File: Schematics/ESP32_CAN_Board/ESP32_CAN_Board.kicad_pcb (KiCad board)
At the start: 4 copper layers, 56 x 50 mm, 36 parts, among them J1 Screw_Terminal_01x04, J2 Screw_Terminal_01x04, J3 Screw_Terminal_01x02, J8 USB_C_Receptacle, U1 SN65HVD230, U4 ESP32-C3-MINI-1-N4, U7 LDL1117-3.3

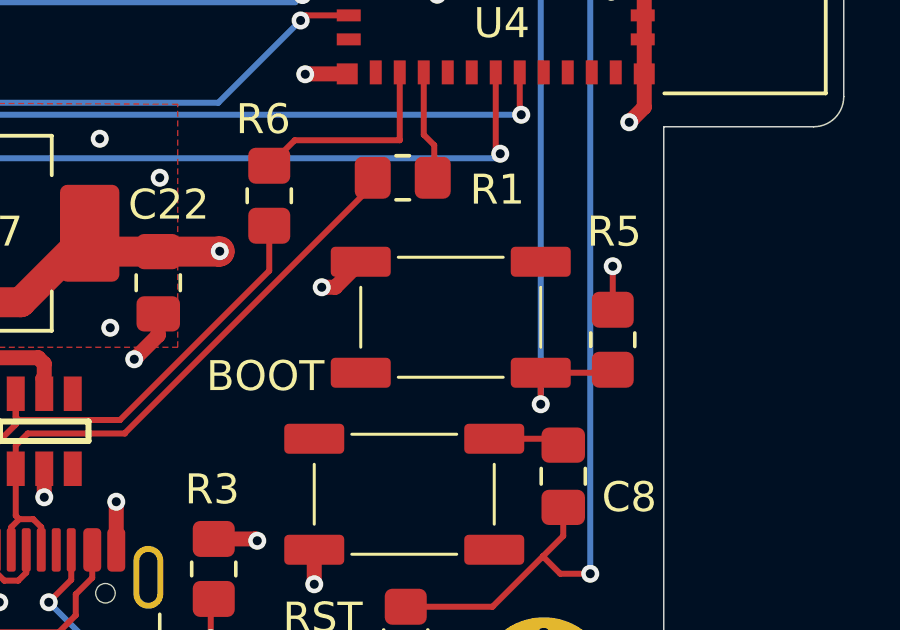
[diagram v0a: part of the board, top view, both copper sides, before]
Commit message: updated ESPBoard
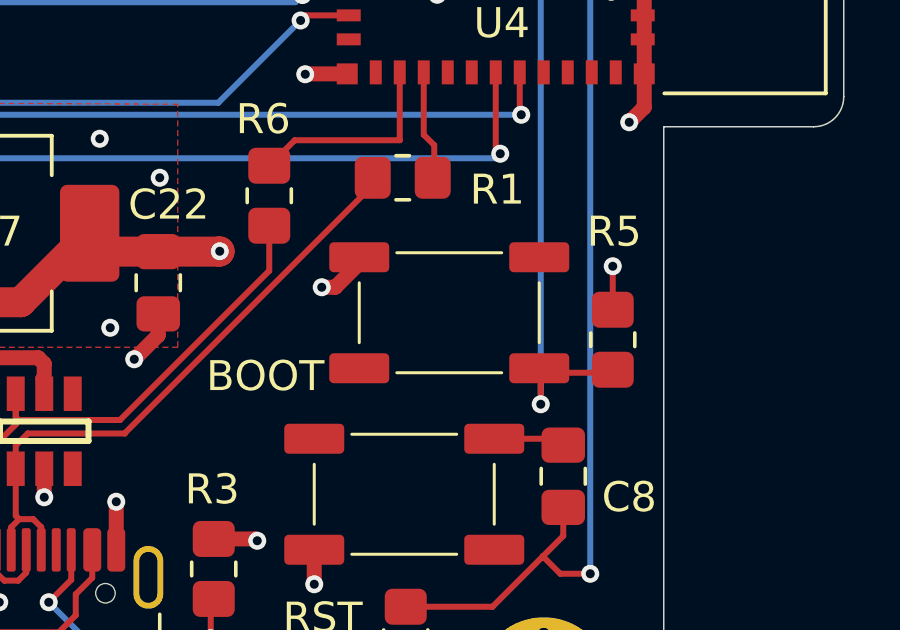
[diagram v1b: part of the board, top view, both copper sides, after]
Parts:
- moved BootSwitch1 0.16 mm to (142.8, 83.6)
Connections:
- BootSwitch1 pad 1: +3.3V -> GND
- R5 pad 1: GND -> +3.3V
- RSTSwitch1 pad 1: unconnected-(RSTSwitch1-Pad1) -> GND
- RSTSwitch1 pad 2: Net-(C8-Pad2) -> unconnected-(RSTSwitch1-Pad2)
- RSTSwitch1 pad 3: GND -> unconnected-(RSTSwitch1-Pad3)
- RSTSwitch1 pad 4: unconnected-(RSTSwitch1-Pad4) -> Net-(C8-Pad2)
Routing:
- net unconnected-(RSTSwitch1-Pad3): track 0.00 -> 1.15 mm, vias 0 -> 1
- net GND: track 71.4 -> 70.5 mm, vias 28 -> 27
